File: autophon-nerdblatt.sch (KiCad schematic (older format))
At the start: 2 parts

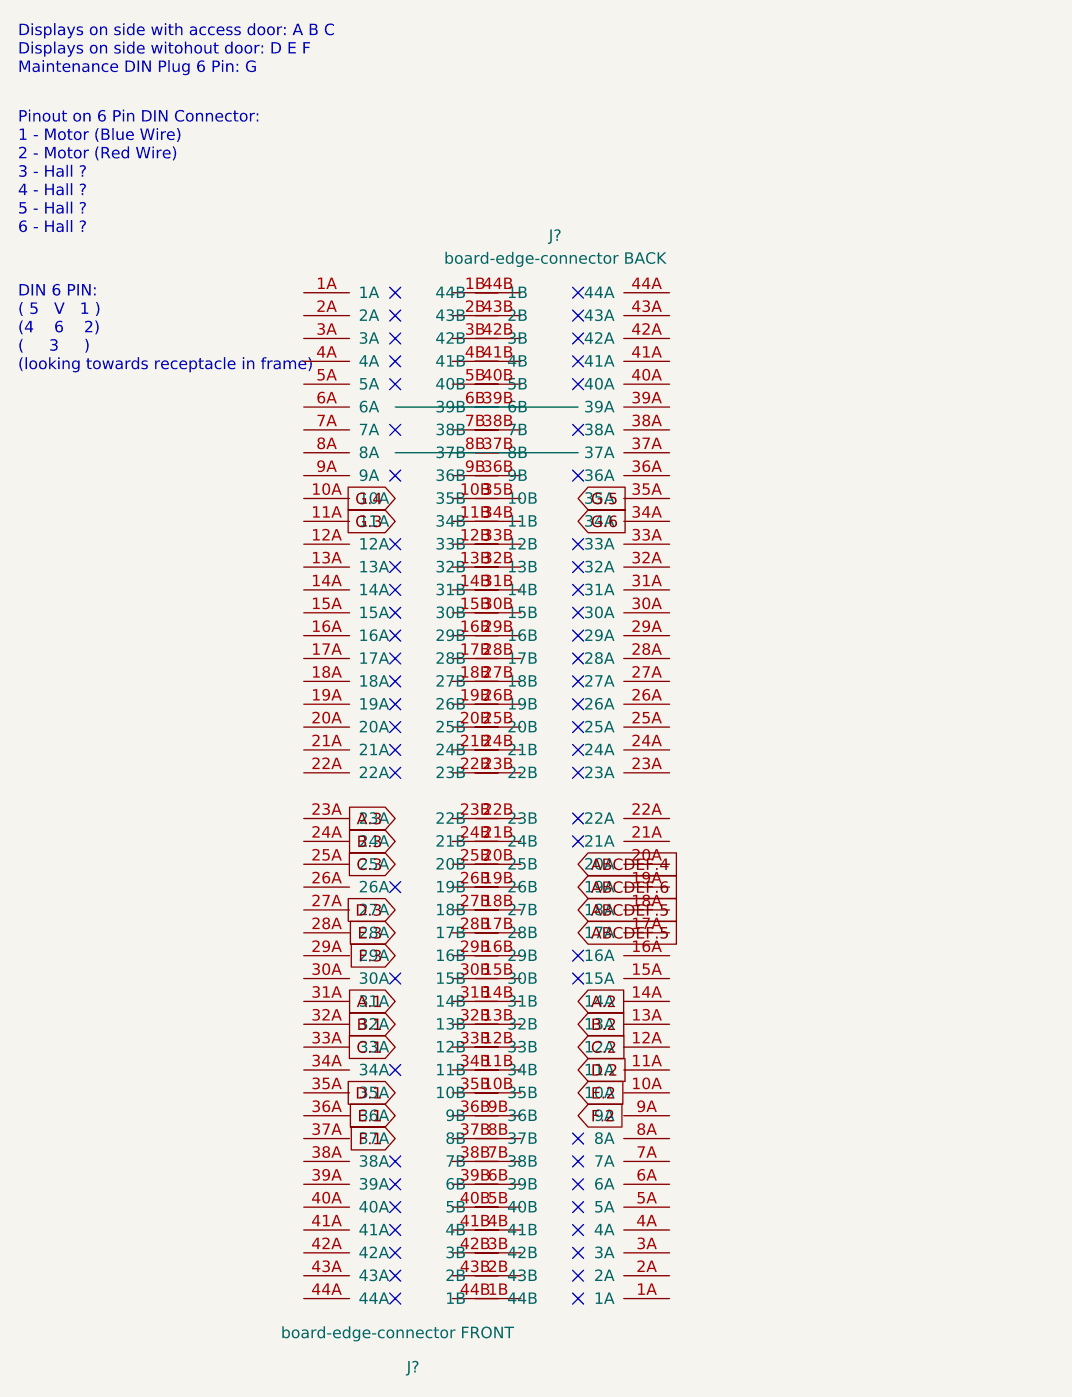
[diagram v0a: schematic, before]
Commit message: Symbol, Footprint improvements. Default Board
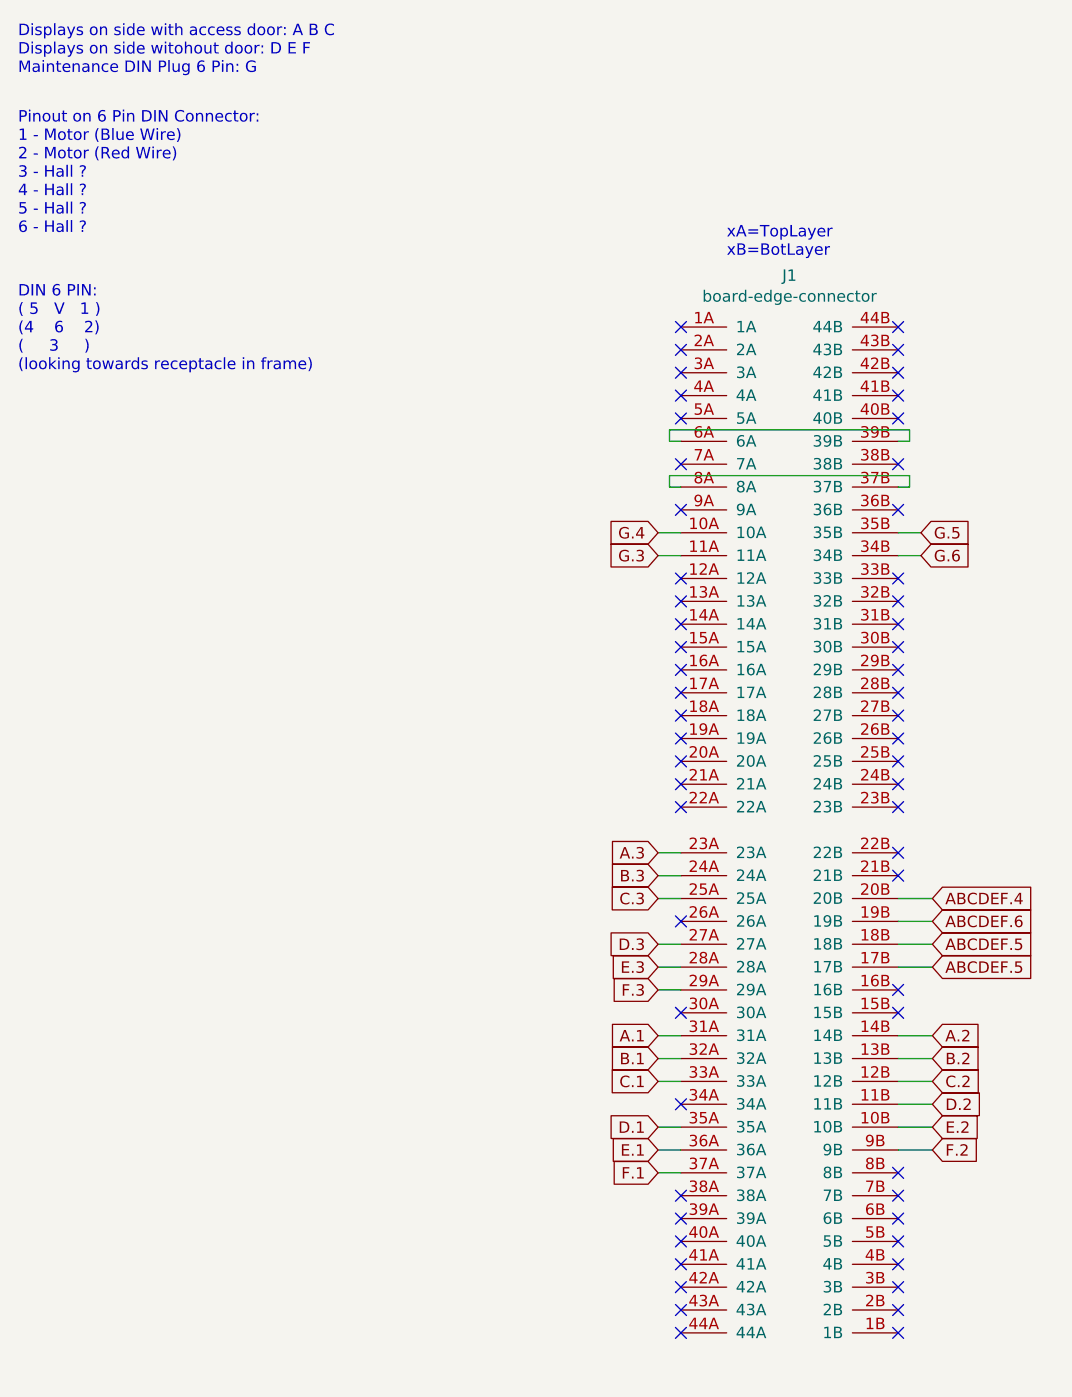
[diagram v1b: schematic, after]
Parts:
- removed J?: board-edge-connector FRONT, symbol autophon-nerdblatt:board-edge-connector
- removed J?: board-edge-connector BACK, symbol autophon-nerdblatt:board-edge-connector
- added J1: board-edge-connector, autophon-nerdblatt:autophon-pcb-edge-connector, symbol autophon-nerdblatt:board-edge-connector
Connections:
- wire segments 2 -> 36
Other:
- note added: "xA=TopLayer\nxB=BotLayer"
